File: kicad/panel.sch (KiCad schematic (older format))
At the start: 8 parts, among them CON21 Panel1, CON22 Panel2, CON5 AUX, SW1 RESET, U2 SN74HCT245PW

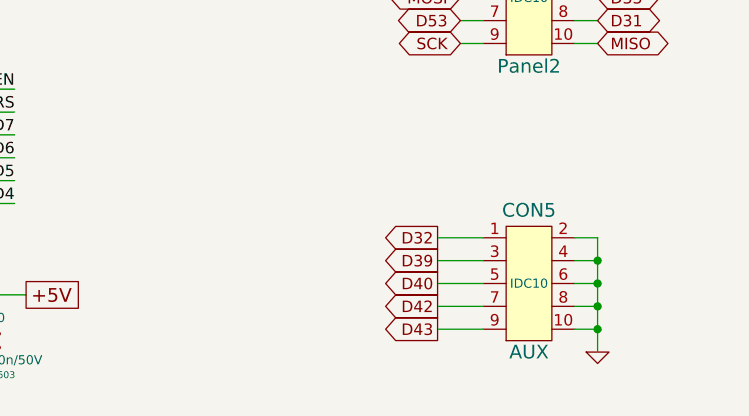
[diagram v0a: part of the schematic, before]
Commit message: Route.
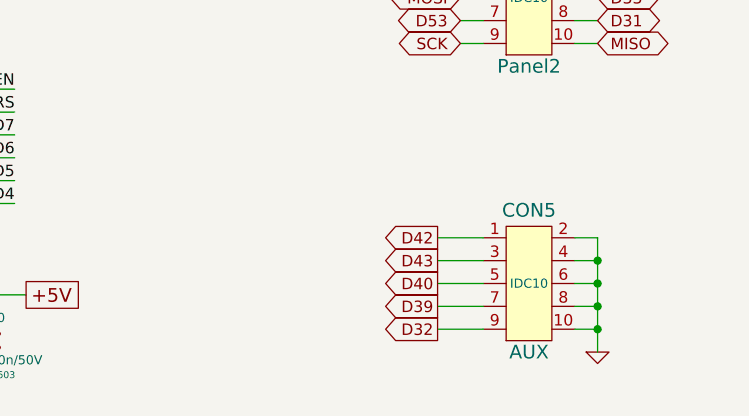
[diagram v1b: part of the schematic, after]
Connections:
- net D32: now also CON5.9; no longer CON5.1
- net D39: now also CON5.7; no longer CON5.3
- net D42: now also CON5.1; no longer CON5.7
- net D43: now also CON5.3; no longer CON5.9
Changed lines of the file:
@@
 	1    0    0    -1
 $EndComp
-Text GLabel 5450 3700 0    50   Output ~ 0
+Text GLabel 5450 4100 0    50   Output ~ 0
 D32
-Text GLabel 5450 3800 0    50   Output ~ 0
+Text GLabel 5450 4000 0    50   Output ~ 0
 D39
 Text GLabel 5450 3900 0    50   Output ~ 0
 D40
-Text GLabel 5450 4000 0    50   Output ~ 0
+Text GLabel 5450 3700 0    50   Output ~ 0
 D42
-Text GLabel 5450 4100 0    50   Output ~ 0
+Text GLabel 5450 3800 0    50   Output ~ 0
 D43
 Wire Wire Line
